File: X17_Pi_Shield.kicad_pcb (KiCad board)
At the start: 2 copper layers, 85 x 56 mm, 20 parts, among them J1 BM04B-GHS-TBT, J19 430450212, J2 BM02B-GHS-TBT, J3 BM02B-GHS-TBT, J4 BM02B-GHS-TBT, J5 BM02B-GHS-TBT, J6 Conn_01x03_Pin, J9 430450612, U1 4754, U10 4754, U2 TPS2117DRLR, U3 INA260AIPW, U8 RASPBERRY_PI_4B_4GB, U9 ISO3086TDW

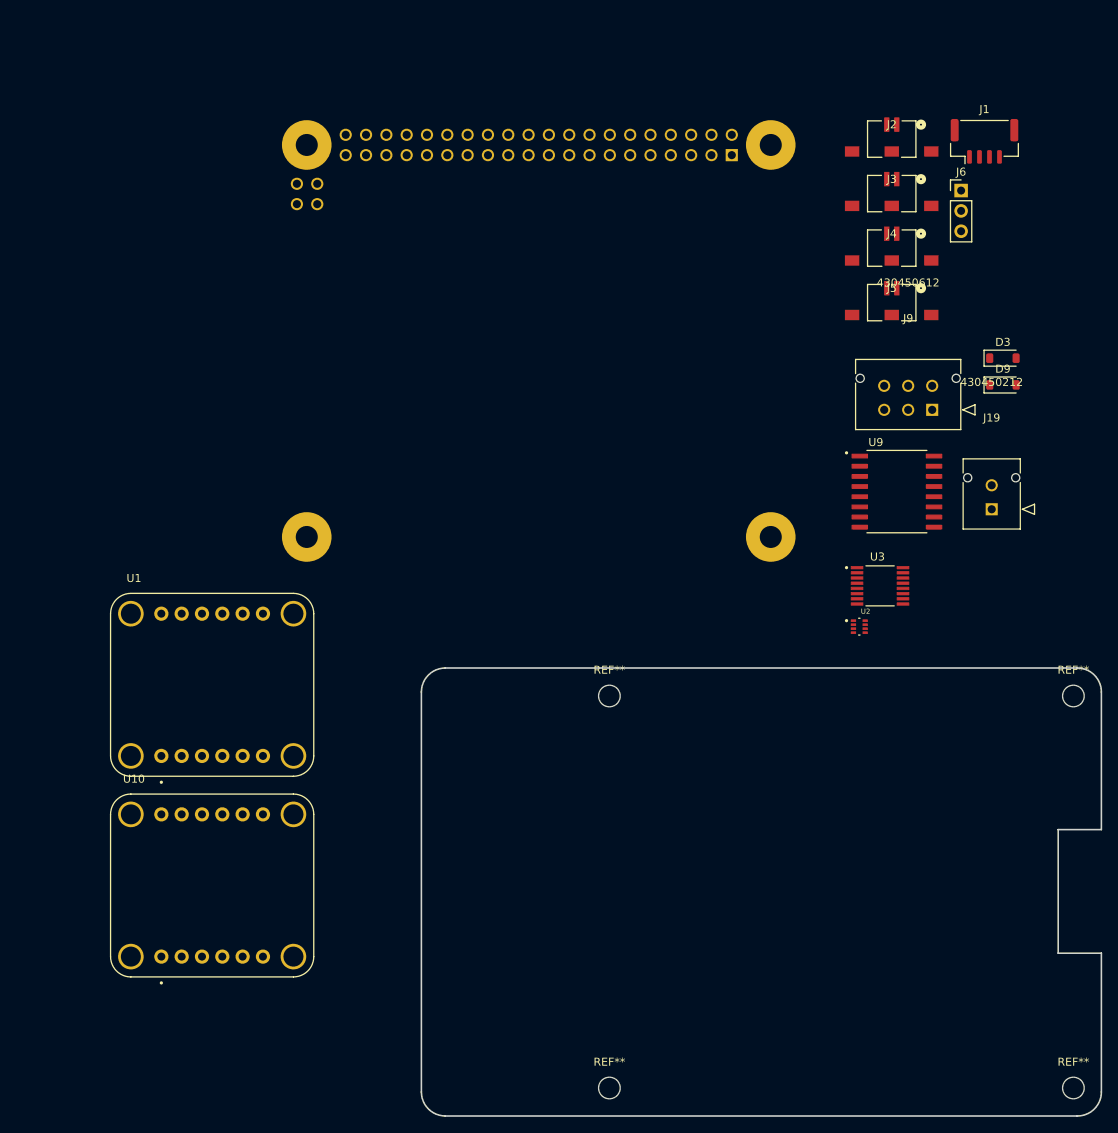
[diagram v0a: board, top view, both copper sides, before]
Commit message: Pre-Toolbox Final
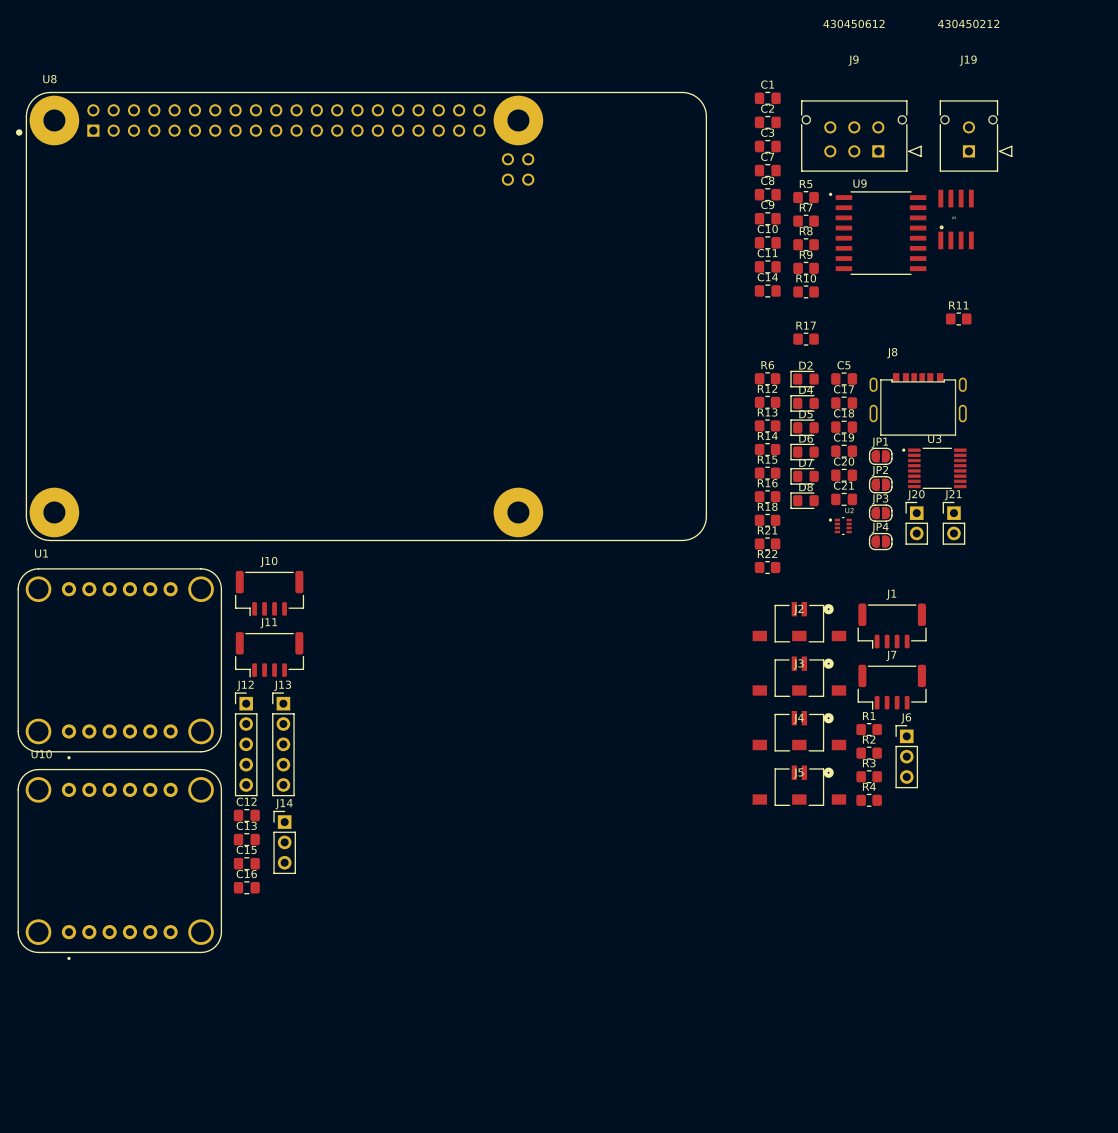
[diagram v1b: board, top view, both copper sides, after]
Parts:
- removed D3, D9: MBR0520LT, Diode_SMD:D_SOD-123
- removed REF** (x4): MountingHole_2.7mm_M2.5_ISO14580, MountingHole:MountingHole_2.7mm_M2.5_ISO14580
- added C1: 10uF, Capacitor_SMD:C_0805_2012Metric_Pad1.18x1.45mm_HandSolder, F.Cu at (157.9, 49.7)
- added C10: 0.1uF, Capacitor_SMD:C_0805_2012Metric_Pad1.18x1.45mm_HandSolder, F.Cu at (157.9, 67.7)
- added C11: 10nF, Capacitor_SMD:C_0805_2012Metric_Pad1.18x1.45mm_HandSolder, F.Cu at (157.9, 70.7)
- added C12: 10uF, Capacitor_SMD:C_0805_2012Metric_Pad1.18x1.45mm_HandSolder, F.Cu at (92.8, 139.3)
- added C13: 10uF, Capacitor_SMD:C_0805_2012Metric_Pad1.18x1.45mm_HandSolder, F.Cu at (92.8, 142.3)
- added C14: 0.1uF, Capacitor_SMD:C_0805_2012Metric_Pad1.18x1.45mm_HandSolder, F.Cu at (157.9, 73.8)
- added C15: 10uF, Capacitor_SMD:C_0805_2012Metric_Pad1.18x1.45mm_HandSolder, F.Cu at (92.8, 145.3)
- added C16: 10uF, Capacitor_SMD:C_0805_2012Metric_Pad1.18x1.45mm_HandSolder, F.Cu at (92.8, 148.3)
- added C17: 150uF, Capacitor_SMD:C_0805_2012Metric_Pad1.18x1.45mm_HandSolder, F.Cu at (167.4, 87.8)
- added C18: 10uF, Capacitor_SMD:C_0805_2012Metric_Pad1.18x1.45mm_HandSolder, F.Cu at (167.4, 90.8)
- added C19: 0.1uF, Capacitor_SMD:C_0805_2012Metric_Pad1.18x1.45mm_HandSolder, F.Cu at (167.4, 93.8)
- added C2: 4.7uF, Capacitor_SMD:C_0805_2012Metric_Pad1.18x1.45mm_HandSolder, F.Cu at (157.9, 52.7)
- added C20: 0.1uF, Capacitor_SMD:C_0805_2012Metric_Pad1.18x1.45mm_HandSolder, F.Cu at (167.4, 96.8)
- added C21: 22uF, Capacitor_SMD:C_0805_2012Metric_Pad1.18x1.45mm_HandSolder, F.Cu at (167.4, 99.8)
- added C3: 10uF, Capacitor_SMD:C_0805_2012Metric_Pad1.18x1.45mm_HandSolder, F.Cu at (157.9, 55.7)
- added C5: 150uF, Capacitor_SMD:C_0805_2012Metric_Pad1.18x1.45mm_HandSolder, F.Cu at (167.4, 84.8)
- added C7: 10uF, Capacitor_SMD:C_0805_2012Metric_Pad1.18x1.45mm_HandSolder, F.Cu at (157.9, 58.7)
- added C8: 0.1uF, Capacitor_SMD:C_0805_2012Metric_Pad1.18x1.45mm_HandSolder, F.Cu at (157.9, 61.7)
- added C9: 4.7uF, Capacitor_SMD:C_0805_2012Metric_Pad1.18x1.45mm_HandSolder, F.Cu at (157.9, 64.7)
- added D2: LED, LED_SMD:LED_0805_2012Metric_Pad1.15x1.40mm_HandSolder, F.Cu at (162.6, 84.8)
- added D4: LED, LED_SMD:LED_0805_2012Metric_Pad1.15x1.40mm_HandSolder, F.Cu at (162.6, 87.8)
- added D5: LED, LED_SMD:LED_0805_2012Metric_Pad1.15x1.40mm_HandSolder, F.Cu at (162.6, 90.8)
- added D6: LED, LED_SMD:LED_0805_2012Metric_Pad1.15x1.40mm_HandSolder, F.Cu at (162.6, 93.9)
- added D7: LED, LED_SMD:LED_0805_2012Metric_Pad1.15x1.40mm_HandSolder, F.Cu at (162.6, 96.9)
- added D8: LED, LED_SMD:LED_0805_2012Metric_Pad1.15x1.40mm_HandSolder, F.Cu at (162.6, 100.0)
- added J10: BM04B-GHS-TBT, Connector_JST:JST_GH_BM04B-GHS-TBT_1x04-1MP_P1.25mm_Vertical, F.Cu at (95.6, 111.5)
- added J11: BM04B-GHS-TBT, Connector_JST:JST_GH_BM04B-GHS-TBT_1x04-1MP_P1.25mm_Vertical, F.Cu at (95.6, 119.2)
- added J12: Conn_01x05_Pin, Connector_PinHeader_2.54mm:PinHeader_1x05_P2.54mm_Vertical, F.Cu at (92.7, 125.3)
- added J13: Conn_01x03_Pin, Connector_PinHeader_2.54mm:PinHeader_1x05_P2.54mm_Vertical, F.Cu at (97.3, 125.3)
- added J14: Conn_01x03_Pin, Connector_PinHeader_2.54mm:PinHeader_1x03_P2.54mm_Vertical, F.Cu at (97.5, 140.1)
- added J20: Conn_01x02_Pin, Connector_PinHeader_2.54mm:PinHeader_1x02_P2.54mm_Vertical, F.Cu at (176.5, 101.5)
- added J21: Conn_01x02_Pin, Connector_PinHeader_2.54mm:PinHeader_1x02_P2.54mm_Vertical, F.Cu at (181.2, 101.5)
- added J7: BM04B-GHS-TBT, Connector_JST:JST_GH_BM04B-GHS-TBT_1x04-1MP_P1.25mm_Vertical, F.Cu at (173.4, 123.3)
- added J8: UJC-HP-L-G-5-MSMT-TR, UJC_HP_L_G_5_MSMT_TR:CUI_UJC-HP-L-G-5-MSMT-TR, F.Cu at (176.7, 89.1)
- added JP1: SolderJumper_2_Open, Jumper:SolderJumper-2_P1.3mm_Open_RoundedPad1.0x1.5mm, F.Cu at (172.0, 94.4)
- added JP2: SolderJumper_2_Open, Jumper:SolderJumper-2_P1.3mm_Open_RoundedPad1.0x1.5mm, F.Cu at (172.0, 98.0)
- added JP3: SolderJumper_2_Open, Jumper:SolderJumper-2_P1.3mm_Open_RoundedPad1.0x1.5mm, F.Cu at (172.0, 101.5)
- added JP4: SolderJumper_2_Open, Jumper:SolderJumper-2_P1.3mm_Open_RoundedPad1.0x1.5mm, F.Cu at (172.0, 105.1)
- added R1: 1K, Resistor_SMD:R_0805_2012Metric_Pad1.20x1.40mm_HandSolder, F.Cu at (170.6, 128.6)
- added R10: 10k, Resistor_SMD:R_0805_2012Metric_Pad1.20x1.40mm_HandSolder, F.Cu at (162.7, 73.9)
- added R11: 10k, Resistor_SMD:R_0805_2012Metric_Pad1.20x1.40mm_HandSolder, F.Cu at (181.8, 77.2)
- added R12: 240, Resistor_SMD:R_0805_2012Metric_Pad1.20x1.40mm_HandSolder, F.Cu at (157.8, 87.7)
- added R13: 240, Resistor_SMD:R_0805_2012Metric_Pad1.20x1.40mm_HandSolder, F.Cu at (157.8, 90.6)
- added R14: 240, Resistor_SMD:R_0805_2012Metric_Pad1.20x1.40mm_HandSolder, F.Cu at (157.8, 93.6)
- added R15: 240, Resistor_SMD:R_0805_2012Metric_Pad1.20x1.40mm_HandSolder, F.Cu at (157.8, 96.5)
- added R16: 240, Resistor_SMD:R_0805_2012Metric_Pad1.20x1.40mm_HandSolder, F.Cu at (157.8, 99.5)
- added R17: 20k, Resistor_SMD:R_0805_2012Metric_Pad1.20x1.40mm_HandSolder, F.Cu at (162.7, 79.8)
- added R18: 1K, Resistor_SMD:R_0805_2012Metric_Pad1.20x1.40mm_HandSolder, F.Cu at (157.8, 102.4)
- added R2: 27K, Resistor_SMD:R_0805_2012Metric_Pad1.20x1.40mm_HandSolder, F.Cu at (170.6, 131.5)
- added R21: 1K, Resistor_SMD:R_0805_2012Metric_Pad1.20x1.40mm_HandSolder, F.Cu at (157.8, 105.4)
- added R22: 2K, Resistor_SMD:R_0805_2012Metric_Pad1.20x1.40mm_HandSolder, F.Cu at (157.8, 108.3)
- added R3: 1K, Resistor_SMD:R_0805_2012Metric_Pad1.20x1.40mm_HandSolder, F.Cu at (170.6, 134.5)
- added R4: 240, Resistor_SMD:R_0805_2012Metric_Pad1.20x1.40mm_HandSolder, F.Cu at (170.6, 137.4)
- added R5: 10k, Resistor_SMD:R_0805_2012Metric_Pad1.20x1.40mm_HandSolder, F.Cu at (162.7, 62.1)
- added R6: 240, Resistor_SMD:R_0805_2012Metric_Pad1.20x1.40mm_HandSolder, F.Cu at (157.8, 84.7)
- added R7: 10k, Resistor_SMD:R_0805_2012Metric_Pad1.20x1.40mm_HandSolder, F.Cu at (162.7, 65.0)
- added R8: 10k, Resistor_SMD:R_0805_2012Metric_Pad1.20x1.40mm_HandSolder, F.Cu at (162.7, 68.0)
- added R9: 20k, Resistor_SMD:R_0805_2012Metric_Pad1.20x1.40mm_HandSolder, F.Cu at (162.7, 70.9)
- added U5: MAX485, MAX485:SO08, F.Cu at (181.4, 64.8)
- U8: moved to F.Cu
- moved J6 68.6 mm to (175.2, 129.4)
- moved J1 61.7 mm to (173.4, 115.6)
- moved J2 61.7 mm to (161.8, 115.3)
- moved J4 61.7 mm to (161.8, 129.0)
- moved J5 61.7 mm to (161.8, 135.8)
- moved J3 61.7 mm to (161.8, 122.1)
- moved J19 44.8 mm to (183.0, 56.3)
- moved J9 33.0 mm to (171.7, 56.3)
- moved U9 32.4 mm to (172.0, 66.5)
- moved U3 16.3 mm to (179.1, 95.9)
- moved U2 12.7 mm to (167.3, 103.1)
- moved U1 11.9 mm to (76.9, 119.9)
- moved U10 11.9 mm to (76.9, 145.0)
- moved U8 11.9 mm to (107.7, 76.9), turned to 0 degrees
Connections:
- J1 pad 1: +5V -> +3V3
- U1 pad JP1_2: +3V3 -> unconnected-(U1-3VO-PadJP1_2)
- U10 pad JP1_2: +3V3 -> unconnected-(U10-3VO-PadJP1_2)
- U2 pad 7: /Power/5V_TOTAL -> unconnected-(U2-VOUT__1-Pad7)
- U8 pad 16: unconnected-(U8-GPIO23/GPIO_GEN4-Pad16) -> /Pi + IMU/LEAK
- U8 pad 26: /Pi + IMU/CE1 -> unconnected-(U8-GPIO7/~{SPI_CE1}-Pad26)
- U8 pad 32: /Pi + IMU/BKP_EN -> /Pi + IMU/TX_TB
- U8 pad 33: /Pi + IMU/TB_EN -> /Pi + IMU/RX_TB
- U8 pad 35: /Pi + IMU/LEAK -> /Pi + IMU/BKP_EN
- U8 pad 38: unconnected-(U8-GPIO20-Pad38) -> /Pi + IMU/TB_EN
- U8 pad S1: Net-(U8-SHIELD-PadS1) -> unconnected-(U8-SHIELD-PadS1)
- U8 pad S2: Net-(U8-SHIELD-PadS1) -> unconnected-(U8-SHIELD-PadS1)_2
- U8 pad S3: Net-(U8-SHIELD-PadS1) -> unconnected-(U8-SHIELD-PadS1)_1
- U8 pad S4: Net-(U8-SHIELD-PadS1) -> unconnected-(U8-SHIELD-PadS1)_3
- U9 pad 16: GND_TB -> Net-(U6-VOUT)
- U9 pad 5: /Pi + IMU/RX -> /Pi + IMU/RX_TB
- U9 pad 8: /Pi + IMU/TX -> /Pi + IMU/TX_TB
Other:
- board size 85 x 56 mm -> 9.3 x 6.9 mm
